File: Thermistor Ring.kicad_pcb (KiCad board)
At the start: 2 copper layers, 48.3 x 48.3 mm, 18 parts, among them J1 Conn_01x04_Socket, U1 TPS7A2018PDBVR, U2 MCP9808T-E/MC, U3 MCP9808T-E/MC, U4 MCP9808T-E/MC, U5 MCP9808T-E/MC, U6 MCP9808T-E/MC, U7 MCP9808T-E/MC

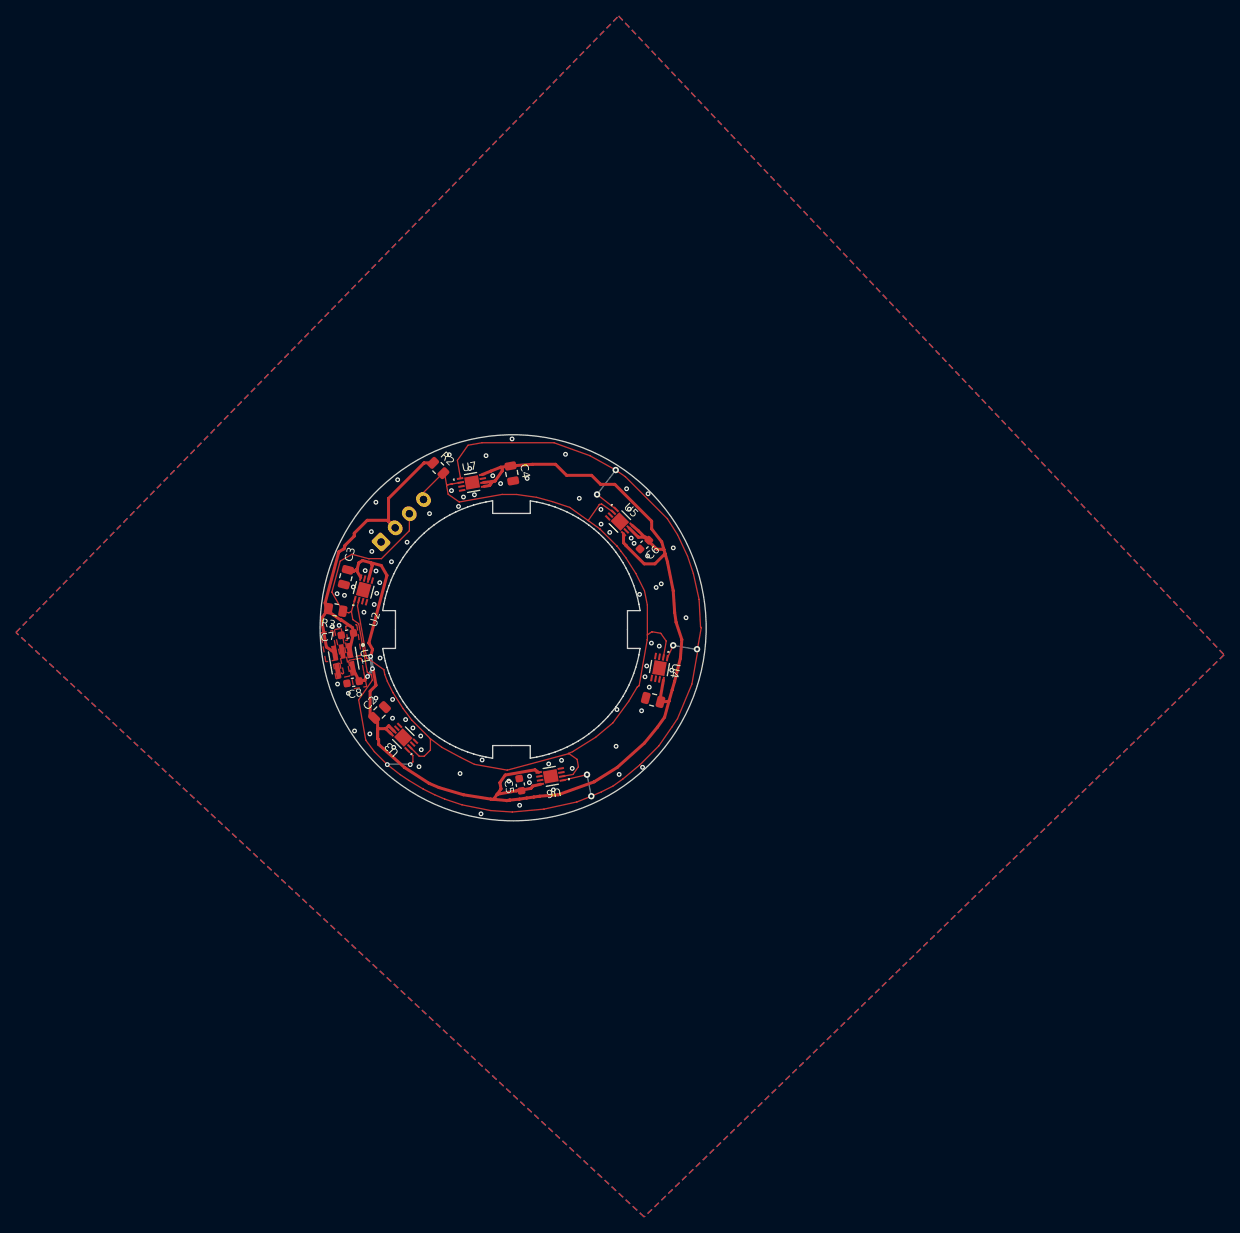
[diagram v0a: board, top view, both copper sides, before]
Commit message: Cleanup
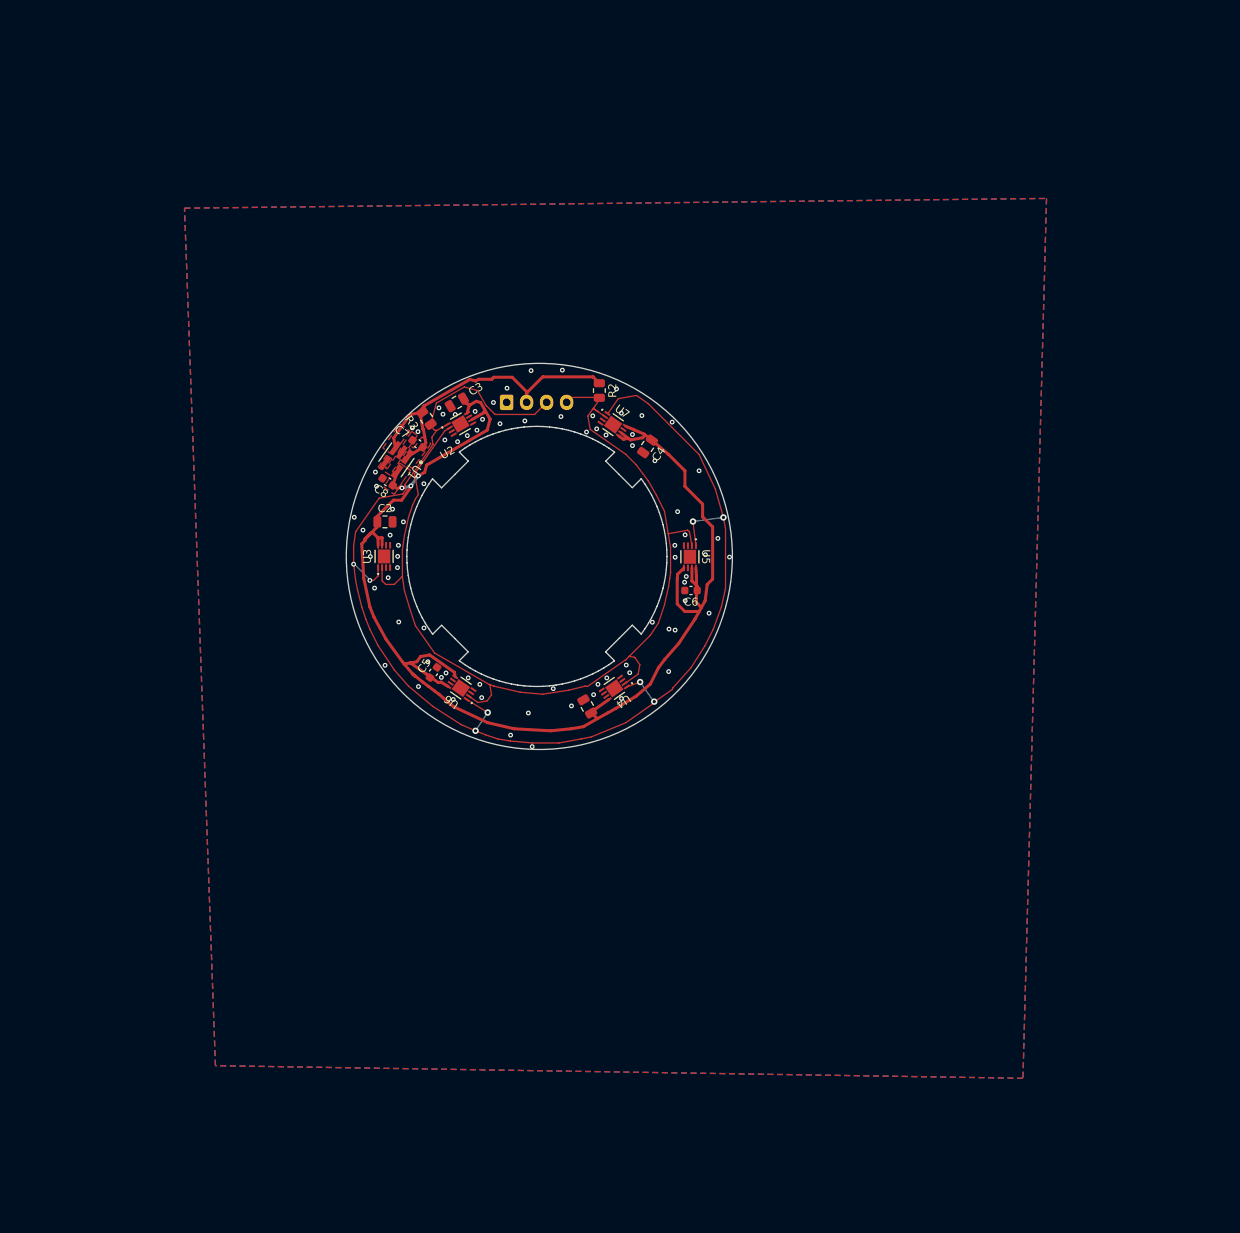
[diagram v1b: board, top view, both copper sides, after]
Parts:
- moved R3 26.5 mm to (62.0, 38.1), turned to -55 degrees
- moved U1 25.9 mm to (58.2, 43.3), turned to -125 degrees
- moved C3 25.9 mm to (65.8, 36.1), turned to -150 degrees
- moved C8 25.4 mm to (57.1, 46.0), turned to 145 degrees
- moved C7 25.4 mm to (60.9, 41.3), turned to 145 degrees
- moved U2 24.0 mm to (66.2, 38.8), turned to 30 degrees
- moved C2 23.8 mm to (56.8, 51.0), turned to 0 degrees
- moved J1 23.5 mm to (72.0, 36.1), turned to 0 degrees
- moved U3 22.8 mm to (56.7, 55.3), turned to 90 degrees
- moved R2 22.3 mm to (83.6, 34.6), turned to -90 degrees
- moved U7 19.0 mm to (85.3, 38.9), turned to -35 degrees
- moved C5 17.7 mm to (62.9, 69.9), turned to 55 degrees
- moved C4 17.3 mm to (89.6, 41.6), turned to -125 degrees
- moved U6 15.7 mm to (66.3, 71.8), turned to 145 degrees
- moved U5 9.80 mm to (94.9, 55.4), turned to -90 degrees
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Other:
- outline, holes or cut-outs redrawn

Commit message: Add fiducials
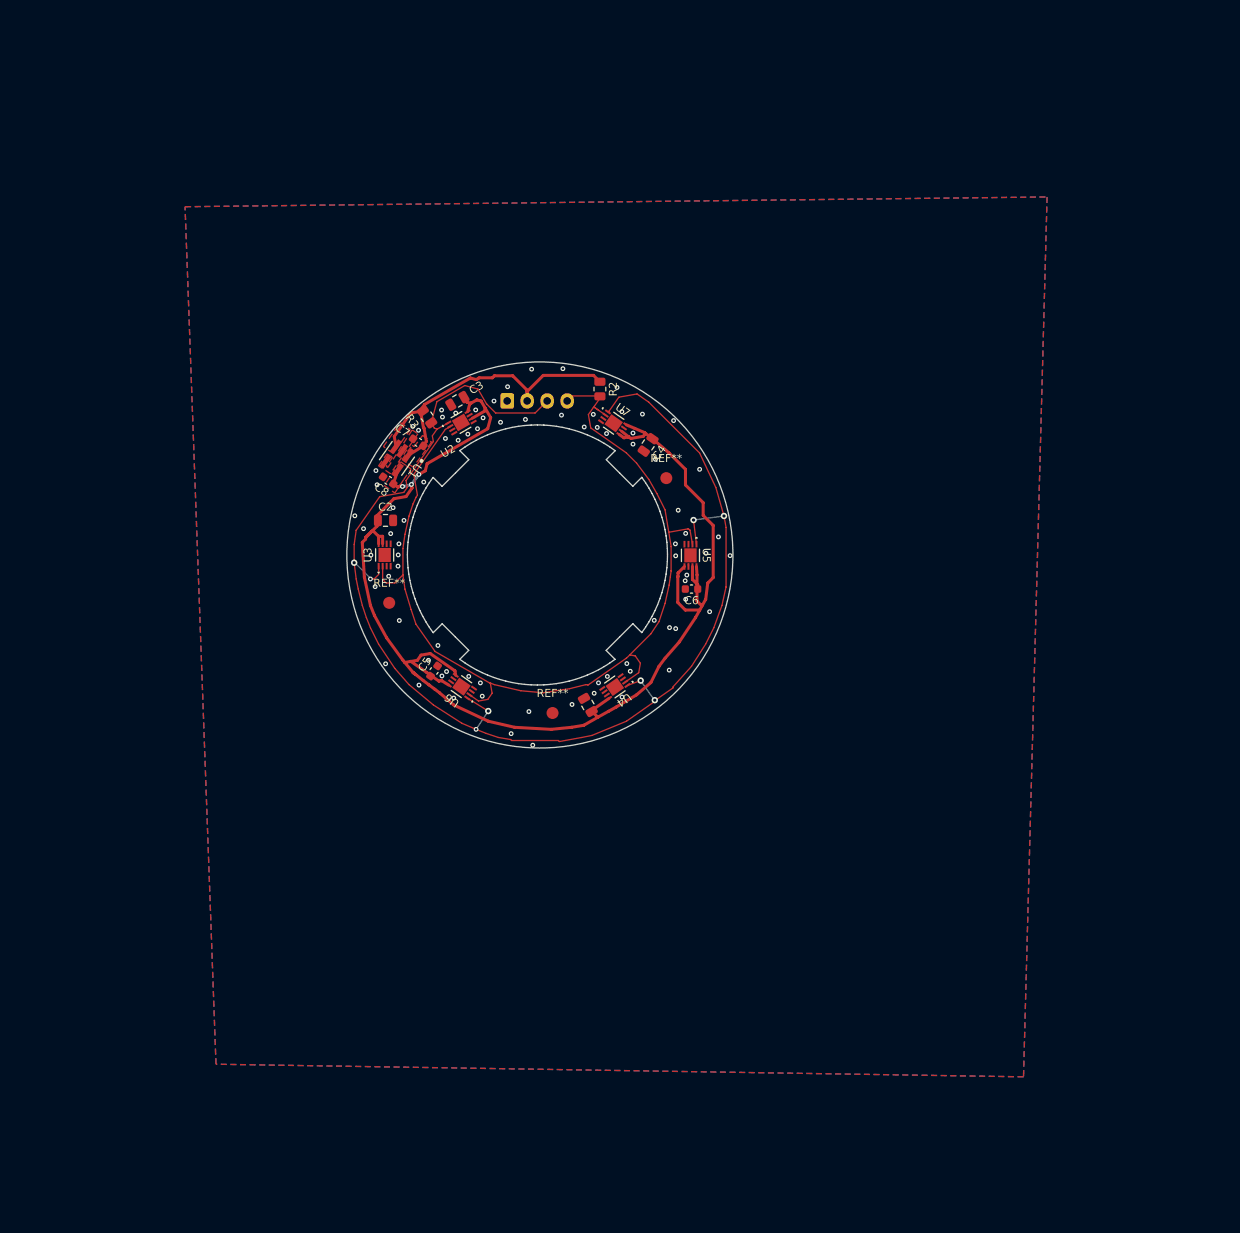
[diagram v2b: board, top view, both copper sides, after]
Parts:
- added REF**: Fiducial_1.5mm_Mask3mm, Fiducial:Fiducial_1.5mm_Mask3mm, F.Cu at (57.3, 61.2)
- added REF**: Fiducial_1.5mm_Mask3mm, Fiducial:Fiducial_1.5mm_Mask3mm, F.Cu at (92.0, 45.6)
- added REF**: Fiducial_1.5mm_Mask3mm, Fiducial:Fiducial_1.5mm_Mask3mm, F.Cu at (77.8, 74.9)
- moved R2 0.19 mm to (83.7, 34.4)
- moved C3 0.19 mm to (65.9, 35.9)
- moved U2 0.19 mm to (66.3, 38.6)
- moved C8 0.19 mm to (57.2, 45.8)
- moved C6 0.19 mm to (95.1, 59.4)
- moved U5 0.19 mm to (95.0, 55.2)
- moved U4 0.19 mm to (85.6, 71.7)
- moved U3 0.19 mm to (56.8, 55.2)
- moved U6 0.19 mm to (66.4, 71.6)
- moved C4 0.19 mm to (89.7, 41.4)
- moved C5 0.19 mm to (62.9, 69.7)
- moved J1 0.19 mm to (72.1, 35.9)
- moved C1 0.19 mm to (82.2, 73.9)
- moved U1 0.19 mm to (58.3, 43.1)
- moved C7 0.19 mm to (61.0, 41.1)
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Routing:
- net GND: vias 81 -> 80
